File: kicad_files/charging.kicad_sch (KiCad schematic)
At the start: 22 parts, among them Q1 AO3400A, Q2 AO3400A, Q3 AO3401A, Q5 Q_PMOS, U2 BQ24172RGYR, U3 CYPD3177-24LQ

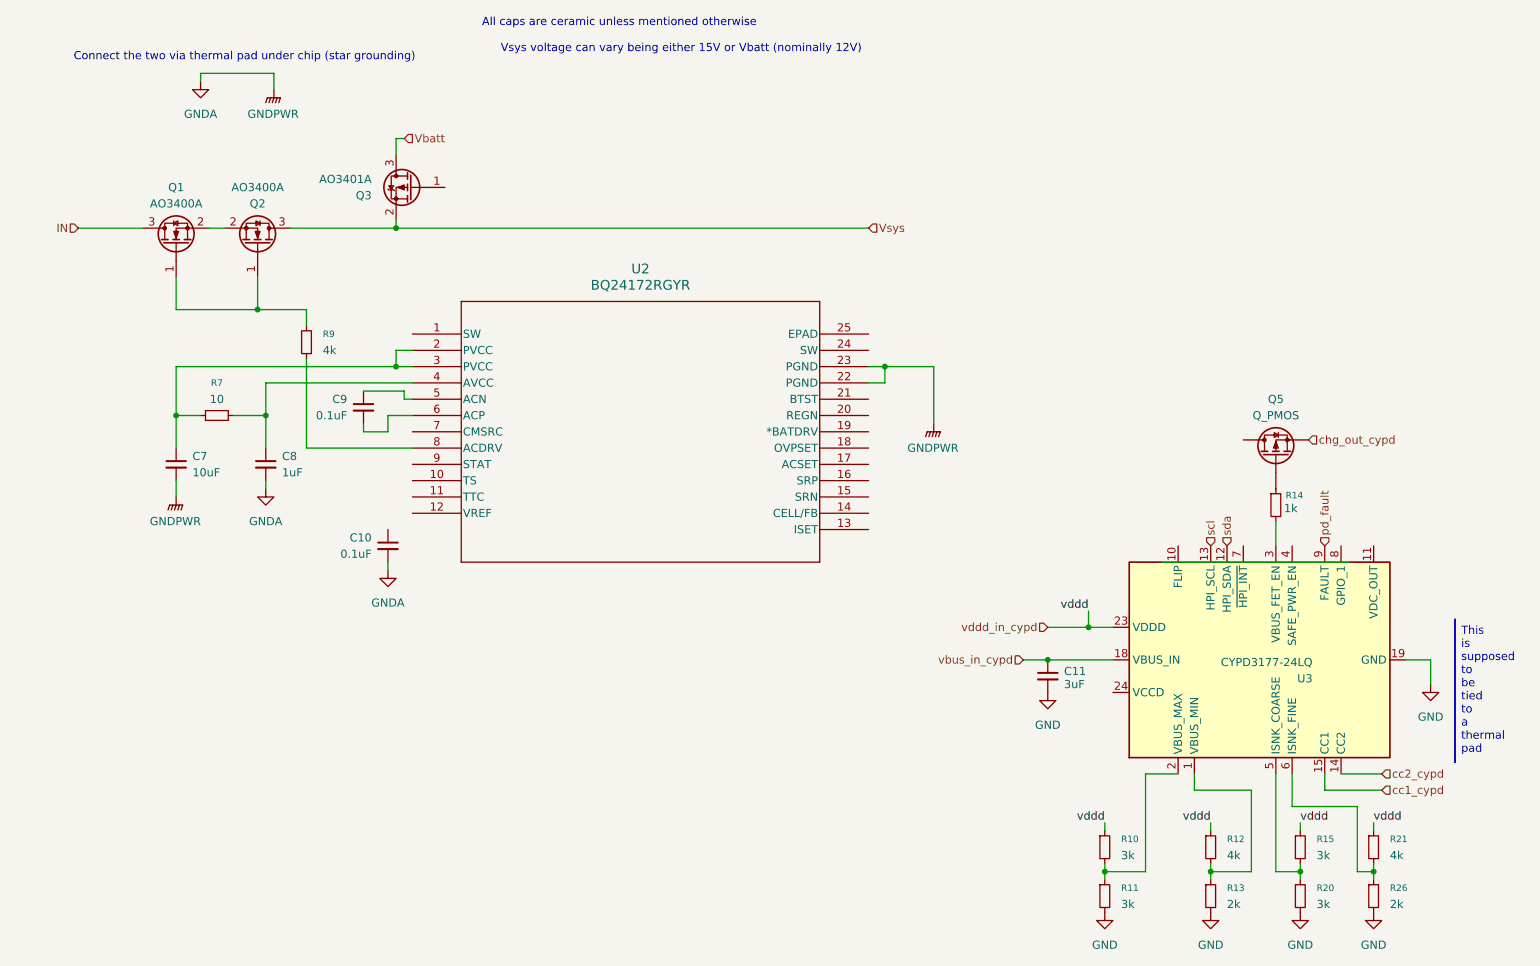
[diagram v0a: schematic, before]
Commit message: A little more progress on BQ24172 IC
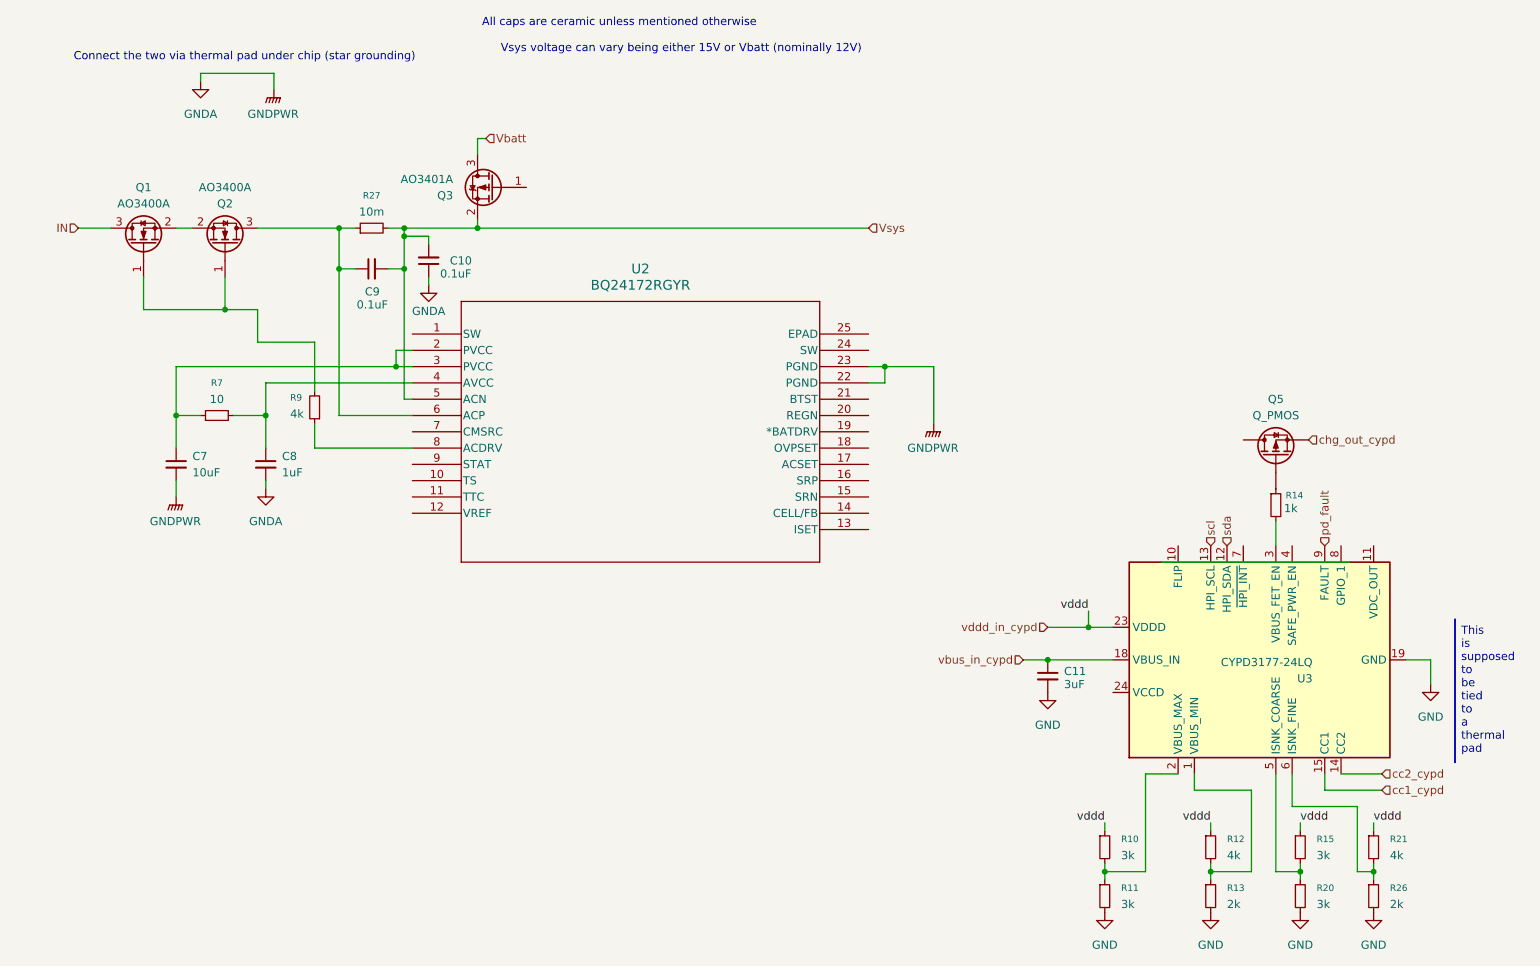
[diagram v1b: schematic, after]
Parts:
- added R27: 10m, symbol Device:R_Small
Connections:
- net GNDA: now also C10.1; no longer C10.2
- net Vsys: now also C10.2, C9.2, U2.5 (ACN), R27.2; no longer Q2.3 (D)
- net at C9.1: now also Q2.3 (D), U2.6 (ACP), R27.1; no longer U2.5 (ACN)
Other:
- moved on the sheet: C10, C9, Q1, Q2, Q3, R9
